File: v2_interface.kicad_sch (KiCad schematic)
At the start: 39 parts, among them J10 Vref_Select, J11 AnalogIO, J12 AUX_Select, J13 DB25_Socket, J14 I^{2}C_TP1, J15 I^{2}C_TP2, J16 SPI_TP1, J17 SPI_TP2, J18 3P_TempSensor, J19 TP, J20 CS_TP, J21 ModPower, J22 5V_PWR, J23 OP_PWR, J8 GAIN_TP, Q1 2N7002K, Q2 2N7002K, U10 MCP3424x-xSL, U8 MCP4922

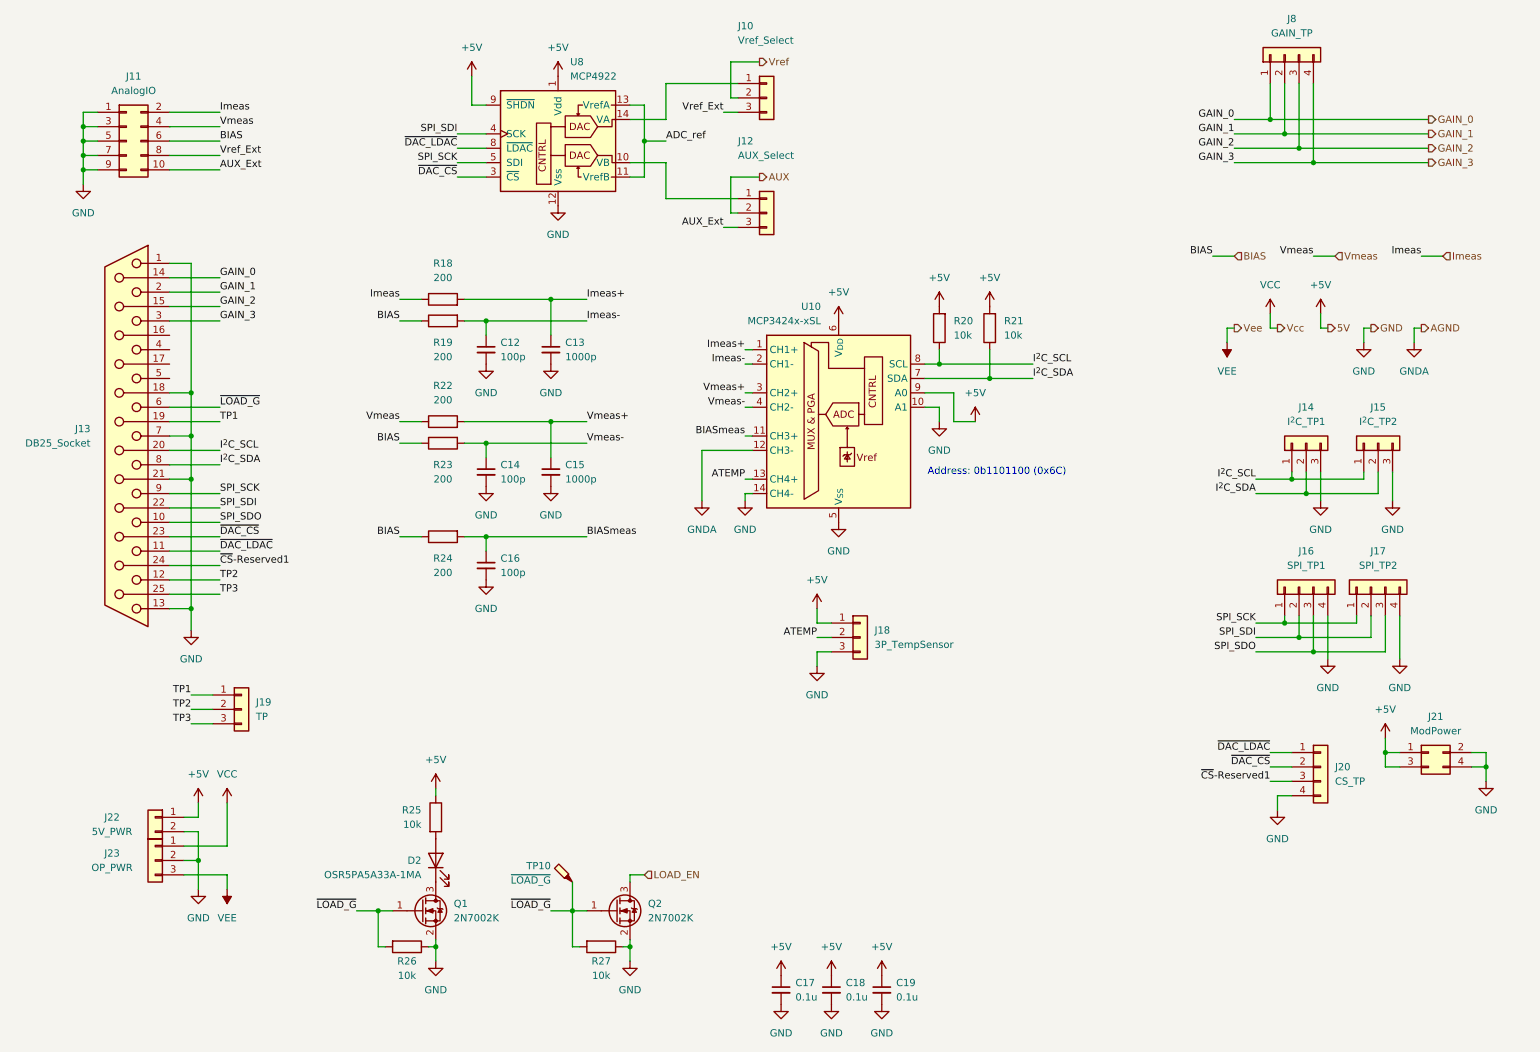
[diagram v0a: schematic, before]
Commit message: 半完成
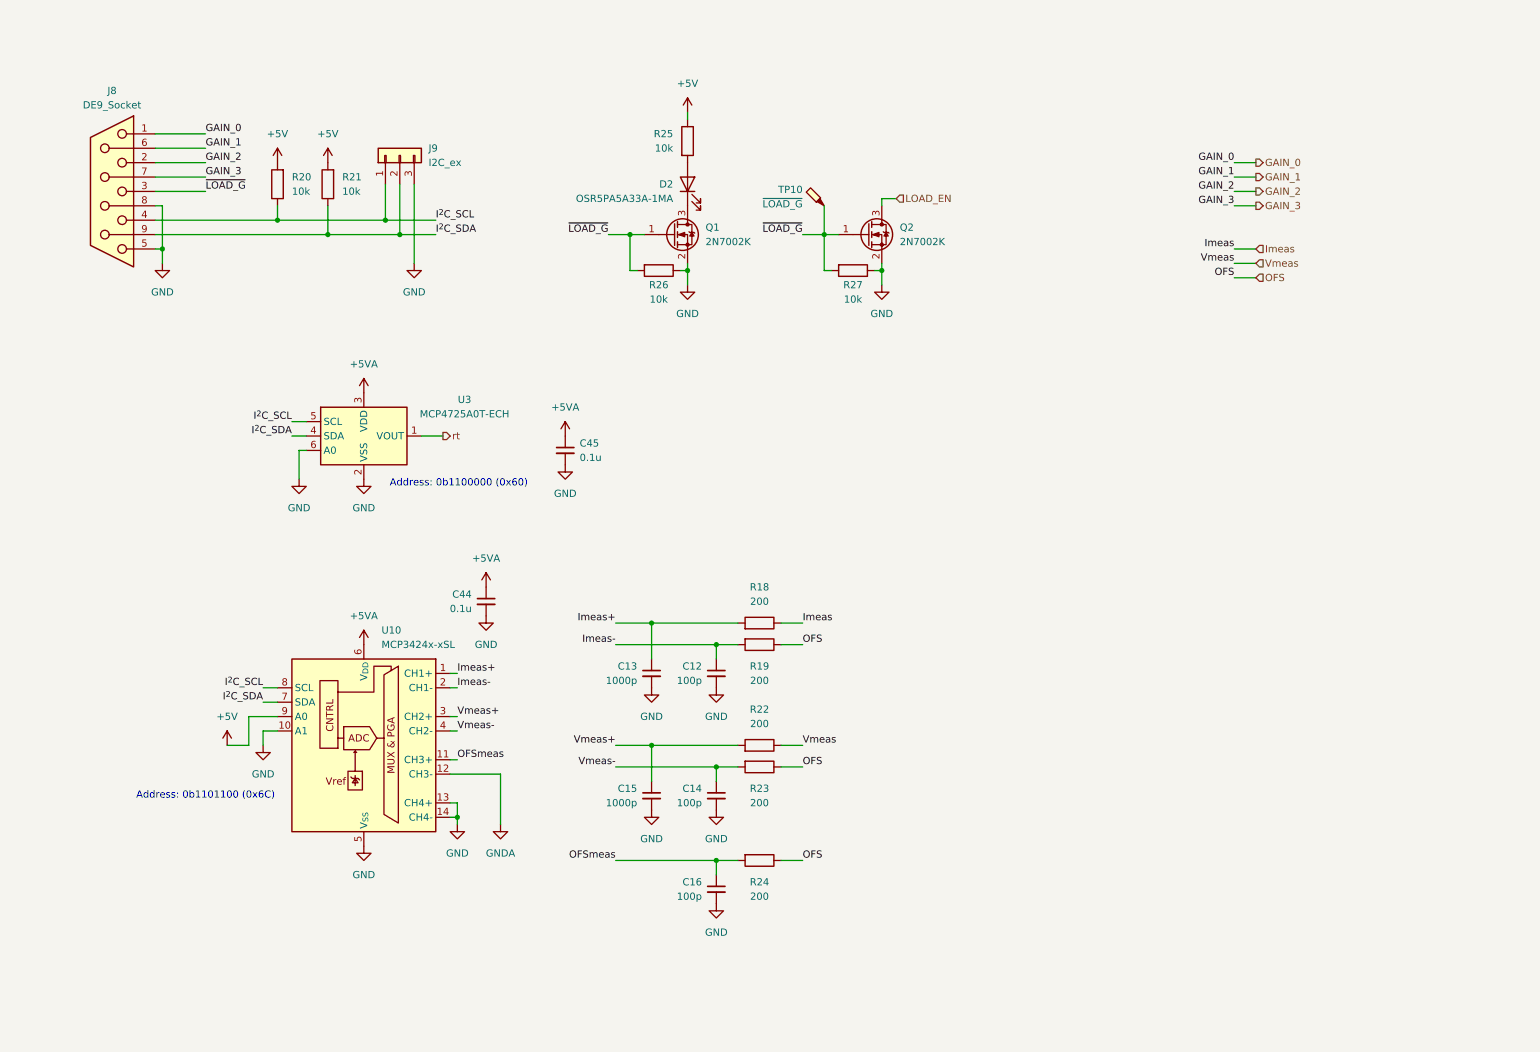
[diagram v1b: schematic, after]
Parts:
- removed C17, C18, C19: 0.1u, Capacitor_SMD:C_0603_1608Metric, symbol Device:C_Small
- removed J10: Vref_Select, Connector_PinHeader_2.54mm:PinHeader_1x03_P2.54mm_Vertical, symbol Connector_Generic:Conn_01x03
- removed J11: AnalogIO, Connector_PinHeader_2.54mm:PinHeader_2x05_P2.54mm_Vertical, symbol Connector_Generic:Conn_02x05_Odd_Even
- removed J12: AUX_Select, Connector_PinHeader_2.54mm:PinHeader_1x03_P2.54mm_Vertical, symbol Connector_Generic:Conn_01x03
- removed J13: DB25_Socket, AM_Conn_Dsub:Dsub-25P_2.77mm-2.84mm-8.08mmOffset, symbol Connector:DB25_Socket
- removed J14: I^{2}C_TP1, Connector_PinHeader_2.54mm:PinHeader_1x03_P2.54mm_Vertical, symbol Connector_Generic:Conn_01x03
- removed J15: I^{2}C_TP2, Connector_PinHeader_2.54mm:PinHeader_1x03_P2.54mm_Vertical, symbol Connector_Generic:Conn_01x03
- removed J16: SPI_TP1, Connector_PinHeader_2.54mm:PinHeader_1x04_P2.54mm_Vertical, symbol Connector_Generic:Conn_01x04
- removed J17: SPI_TP2, Connector_PinHeader_2.54mm:PinHeader_1x04_P2.54mm_Vertical, symbol Connector_Generic:Conn_01x04
- removed J18: 3P_TempSensor, Connector_PinSocket_2.54mm:PinSocket_1x03_P2.54mm_Vertical, symbol Connector_Generic:Conn_01x03
- removed J19: TP, Connector_PinHeader_2.54mm:PinHeader_1x03_P2.54mm_Vertical, symbol Connector_Generic:Conn_01x03
- removed J20: CS_TP, Connector_PinHeader_2.54mm:PinHeader_1x04_P2.54mm_Vertical, symbol Connector_Generic:Conn_01x04
- removed J21: ModPower, Connector_PinHeader_2.00mm:PinHeader_2x02_P2.00mm_Vertical, symbol Connector_Generic:Conn_02x02_Odd_Even
- removed J22: 5V_PWR, AM_Conn_ScrewTerminal:EurostylePluggable_1x02_P5.08mm, symbol Connector_Generic:Conn_01x02
- removed J23: OP_PWR, AM_Conn_ScrewTerminal:EurostylePluggable_1x03_P5.08mm, symbol Connector_Generic:Conn_01x03
- removed J8: GAIN_TP, Connector_PinHeader_2.54mm:PinHeader_1x04_P2.54mm_Vertical, symbol Connector_Generic:Conn_01x04
- removed U8: MCP4922, Package_DIP:DIP-14_W7.62mm, symbol Analog_DAC:MCP4922
- added C44, C45: 0.1u, Capacitor_SMD:C_0603_1608Metric, symbol Device:C_Small
- added J8: DE9_Socket, symbol Connector:DE9_Socket
- added J9: I2C_ex, symbol Connector_Generic:Conn_01x03
- added U3: MCP4725A0T-ECH, Package_TO_SOT_SMD:SOT-23-6, symbol Analog_DAC:MCP4725xxx-xCH
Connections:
- net ATEMP is gone; now on net GND: U10.13 (CH4+)
- net +5V: no longer U10.6 (V_{DD})
- net GAIN_0: now also J8.1
- net GAIN_1: now also J8.6
- net GAIN_2: now also J8.2
- net GAIN_3: now also J8.7
- net GND: now also C44.2, C45.2, J8.5, J8.8, J9.3 (Pin_3), U3.2 (VSS), U3.6 (A0)
- net I^{2}C_SCL: now also J8.4, J9.1 (Pin_1), U3.5 (SCL)
- net I^{2}C_SDA: now also J8.9, J9.2 (Pin_2), U3.4 (SDA)
- net ~{LOAD_G}: now also J8.3
- net BIAS renamed OFS
- net BIASmeas renamed OFSmeas
- new net +5VA: C44.1, C45.1, U10.6 (V_{DD}), U3.3 (VDD)
- new net rt: U3.1 (VOUT)
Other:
- note added: "Address: 0b1100000 (0x60)"
- moved on the sheet: C12, C13, C14, C15, C16, D2, Q1, Q2, R18, R19, R22, R23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

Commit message: aaaa
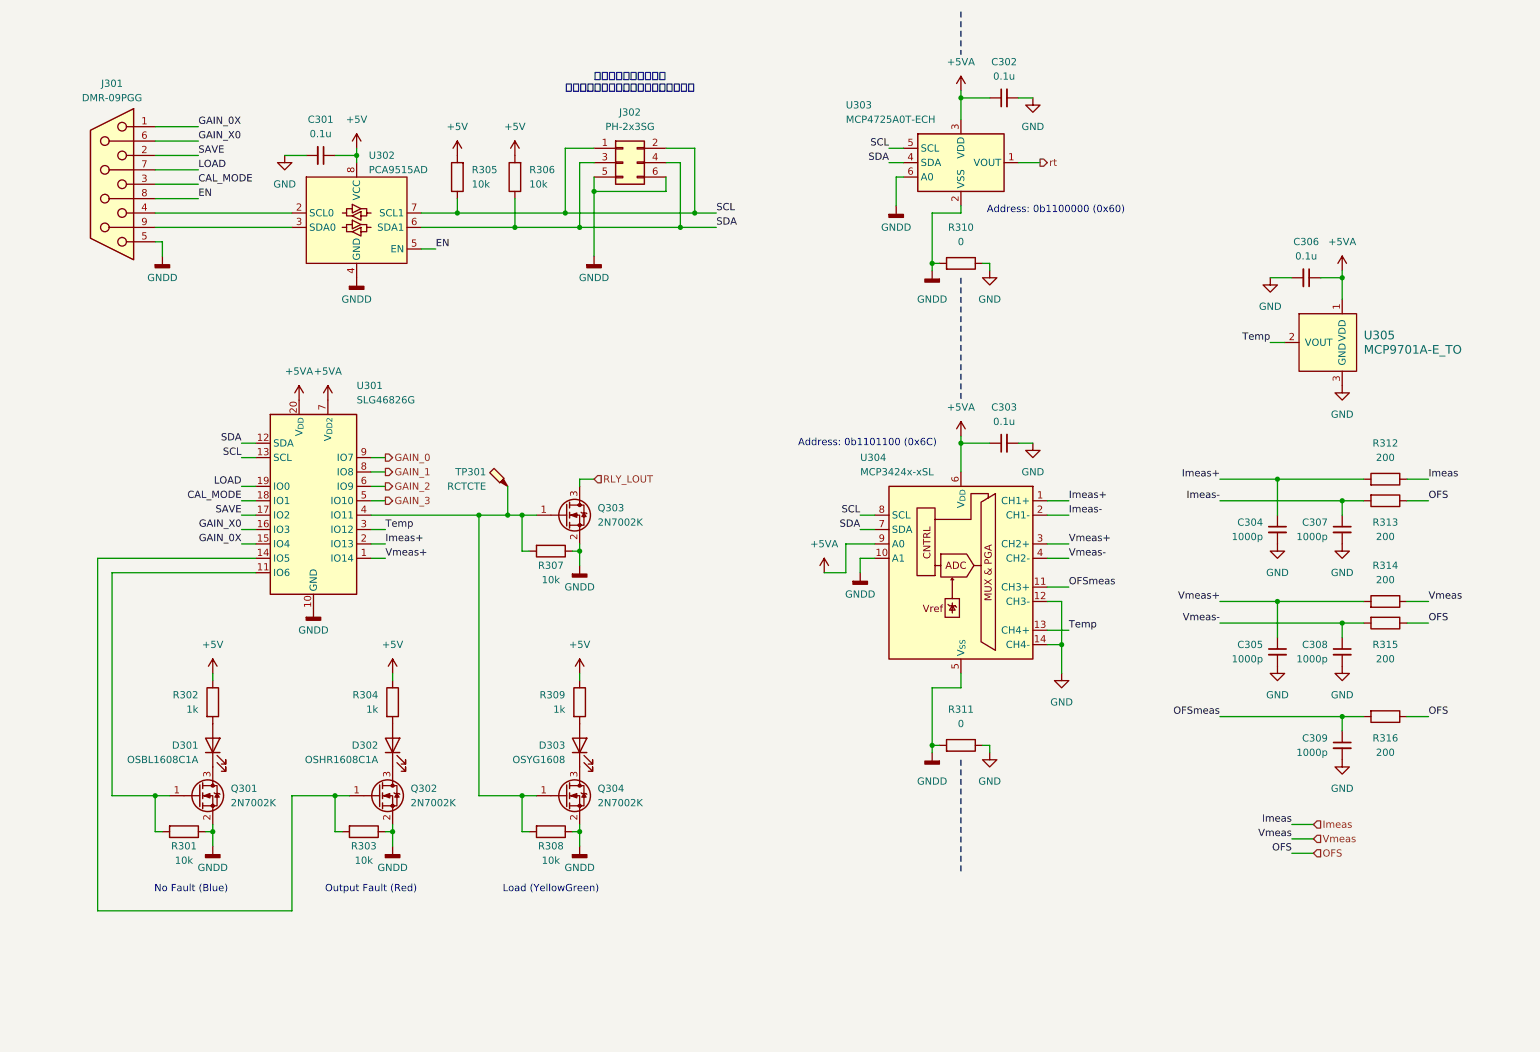
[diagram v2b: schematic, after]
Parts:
- removed C44, C45: 0.1u, Capacitor_SMD:C_0603_1608Metric, symbol Device:C_Small
- removed J9: I2C_ex, symbol Connector_Generic:Conn_01x03
- removed Q2: 2N7002K, Package_TO_SOT_SMD:SOT-23, symbol Transistor_FET:2N7002K
- removed R27: 10k, Resistor_SMD:R_0603_1608Metric, symbol Device:R
- removed TP10: ~{LOAD_G}, TestPoint:TestPoint_Loop_D2.50mm_Drill1.0mm, symbol Connector:TestPoint_Probe
- added C301, C302, C303, C306: 0.1u, Capacitor_SMD:C_0603_1608Metric, symbol Device:C_Small
- added D301: OSBL1608C1A, LED_SMD:LED_0603_1608Metric, symbol Device:LED
- added D302: OSHR1608C1A, LED_SMD:LED_0603_1608Metric, symbol Device:LED
- added J302: PH-2x3SG, Connector_PinHeader_2.54mm:PinHeader_2x03_P2.54mm_Vertical, symbol Connector_Generic:Conn_02x03_Odd_Even
- added Q301, Q302, Q303: 2N7002K, Package_TO_SOT_SMD:SOT-23, symbol Transistor_FET:2N7002K
- added R301, R303, R307: 10k, Resistor_SMD:R_0603_1608Metric, symbol Device:R
- added R302, R304: 1k, Resistor_SMD:R_0603_1608Metric, symbol Device:R
- added R310, R311: 0, Resistor_SMD:R_0805_2012Metric, symbol Device:R
- added TP301: RCTCTE, symbol Connector:TestPoint_Probe
- added U301: SLG46826G, Package_SO:TSSOP-20_4.4x6.5mm_P0.65mm, symbol CPLD_Renesas:SLG46826G
- added U302: PCA9515AD, Package_SO:SOIC-8_3.9x4.9mm_P1.27mm, symbol AM_PLD:PCA9515AD
- added U305: MCP9701A-E_TO, digikey-footprints:TO-92-3, symbol dk_Temperature-Sensors-Analog-and-Digital-Output:MCP9701A-E_TO
- C304: renamed from C13; Akizuki_code (none) -> 102332; Sengoku_code (none) -> EEHD-6WFB
- C305: renamed from C15; Akizuki_code (none) -> 102332; Sengoku_code (none) -> EEHD-6WFB
- C307: renamed from C12; value 100p -> 1000p; Akizuki_code (none) -> 102332; Sengoku_code (none) -> EEHD-6WFB
- C308: renamed from C14; value 100p -> 1000p; Akizuki_code (none) -> 102332; Sengoku_code (none) -> EEHD-6WFB
- C309: renamed from C16; value 100p -> 1000p; Akizuki_code (none) -> 102332; Sengoku_code (none) -> EEHD-6WFB
- D303: renamed from D2; value OSR5PA5A33A-1MA -> OSYG1608; footprint LED_THT:LED_D5.0mm -> LED_SMD:LED_0603_1608Metric; Akizuki_code (none) -> 108275
- J301: renamed from J8; value DE9_Socket -> DMR-09PGG
- R305: renamed from R20; Akizuki_code (none) -> 106668
- R306: renamed from R21; Akizuki_code (none) -> 106668
- R308: renamed from R26; Akizuki_code (none) -> 106668
- R309: renamed from R25; value 10k -> 1k; Akizuki_code (none) -> 10668
- U304: renamed from U10; footprint Package_DIP:DIP-14_W7.62mm -> Package_SO:SOIC-14_3.9x8.7mm_P1.27mm
- renumbered Q1 to Q304, R18 to R312, R19 to R313, R22 to R314, R23 to R315, R24 to R316, U3 to U303
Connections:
- net GNDA is gone; now on net GND: U304.12 (CH3-)
- net +5V: now also C301.1, R302.1, R304.1, U302.8 (VCC); no longer U304.9 (A0)
- net +5VA: now also U304.9 (A0), C302.1, C303.1, C306.1, U301.20 (V_{DD}), U301.7 (V_{DD2}), U305.1 (VDD)
- net GAIN_0: now also U301.9 (IO7); no longer J301.1
- net GAIN_1: now also U301.8 (IO8); no longer J301.6
- net GAIN_2: now also U301.6 (IO9); no longer J301.2
- net GAIN_3: now also U301.5 (IO10); no longer J301.7
- net GND: now also C301.2, C302.2, C303.2, C306.2, R310.1, R311.1, U305.3 (GND); no longer J301.5, J301.8, Q304.2 (S), R308.1, U303.2 (VSS), U303.6 (A0), U304.10 (A1), U304.13 (CH4+), U304.5 (V_{SS})
- net Imeas+: now also U301.2 (IO13)
- net Vmeas+: now also U301.1 (IO14)
- net I^{2}C_SCL renamed SCL
- net SCL: now also J302.1 (Pin_1), J302.2 (Pin_2), U301.13 (SCL), U302.7 (SCL1); no longer J301.4
- net I^{2}C_SDA renamed SDA
- net SDA: now also J302.3 (Pin_3), J302.4 (Pin_4), U301.12 (SDA), U302.6 (SDA1); no longer J301.9
- net ~{LOAD_G}: no longer names the net of Q304.1 (G), R308.2
- net ~{LOAD_G}: now also Q303.1 (G), R307.2, TP301.1, U301.4 (IO11); no longer J301.3
- new net: Q301.1 (G), R301.2, U301.11 (IO6)
- new net: D302.1 (K), Q302.3 (D)
- new net: D302.2 (A), R304.2
- new net: D301.1 (K), Q301.3 (D)
- new net: D301.2 (A), R302.2
- new net: Q302.1 (G), R303.2, U301.14 (IO5)
- new net: J301.4, U302.2 (SCL0)
- new net: J301.9, U302.3 (SDA0)
- new net CAL_MODE: J301.3, U301.18 (IO1)
- new net EN: J301.8, U302.5 (EN)
- new net GAIN_0X: J301.1, U301.15 (IO4)
- new net GAIN_X0: J301.6, U301.16 (IO3)
- new net GNDD: J301.5, J302.5 (Pin_5), J302.6 (Pin_6), Q301.2 (S), Q302.2 (S), Q303.2 (S), Q304.2 (S), R301.1, R303.1, R307.1, R308.1, R310.2, R311.2, U301.10 (GND), U302.4 (GND), U303.2 (VSS), U303.6 (A0), U304.10 (A1), U304.5 (V_{SS})
- new net LOAD: J301.7, U301.19 (IO0)
- new net RLY_LOUT: Q303.3 (D)
- new net SAVE: J301.2, U301.17 (IO2)
- new net Temp: U301.3 (IO12), U304.13 (CH4+), U305.2 (VOUT)
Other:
- note added: "Load (YellowGreen)"
- note added: "No Fault (Blue)"
- note added: "Output Fault (Red)"
- note added: "外付け用兼ロジアナ用 使わないときはジャンパーをつけておく"
- moved on the sheet: C304, C305, C307, C308, C309, D303, J301, Q304, R305, R306, R308, R309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
